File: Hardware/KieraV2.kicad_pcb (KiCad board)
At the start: 2 copper layers, 111 x 63.2 mm, 87 parts, among them J1 Conn_01x04_Male, J2 Conn_01x05_Male, SW1 SW_Rotary2x4, SW2 SW_Rotary2x4, SW3 SW_Push, SW4 SW_Push, SW5 SW_Push, SW6 SW_Push, SW7 SW_MEC_5G, U1 STM32L4P5RET6, U2 LM1117-3.3, U3 IMS330DHCX, U4 ATA6561-GAQW-N, Y1 Crystal_GND24

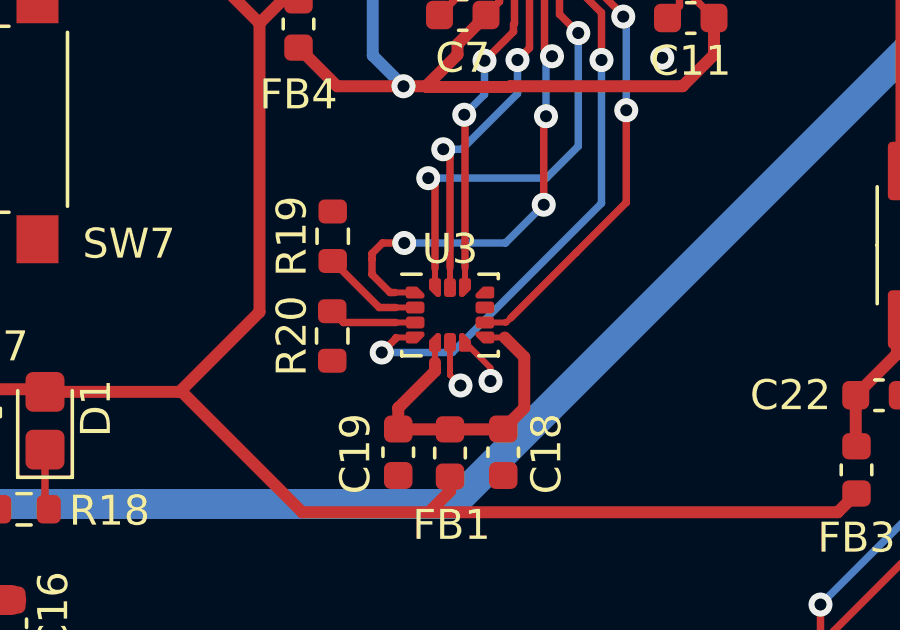
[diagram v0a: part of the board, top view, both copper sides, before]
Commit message: wip
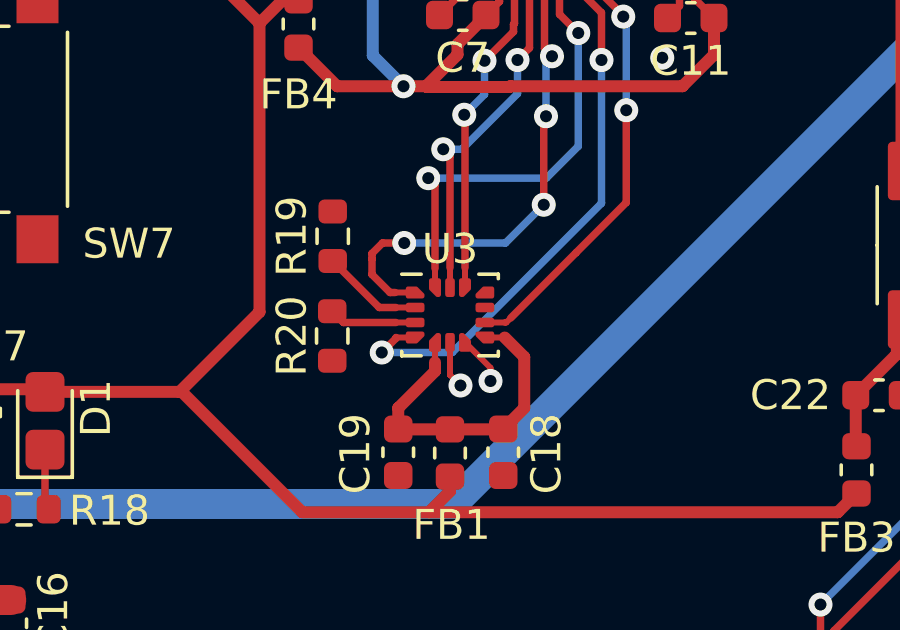
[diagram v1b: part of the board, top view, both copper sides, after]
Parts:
- U3: footprint Package_LGA:LGA-14_3x2.5mm_P0.5mm_LayoutBorder3x4y -> PUTM_Kicad_FOOTPRINTS:LGA-14_3x2.5mm_P0.5mm_LayoutBorder3x4y
